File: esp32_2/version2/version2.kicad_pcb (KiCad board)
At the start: 4 copper layers, 31 x 38.5 mm, 30 parts, among them J1 USB_C_Receptacle_USB2.0_16P, J2 Conn_01x08_Pin, J3 Conn_01x08_Pin, SW1 SW_Push, SW2 SW_Push, U1 USBLC6-2SC6, U2 AP2112K-3.3, U3 ESP32-C3-WROOM-02, Y1 Crystal

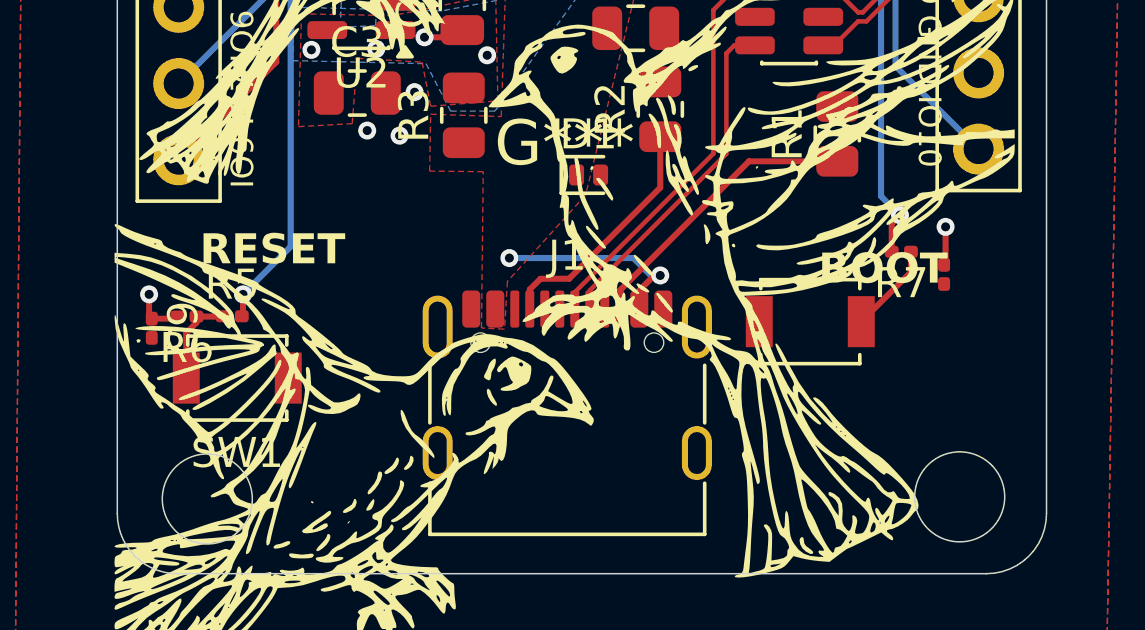
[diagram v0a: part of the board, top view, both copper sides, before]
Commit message: oops some formatting stuff
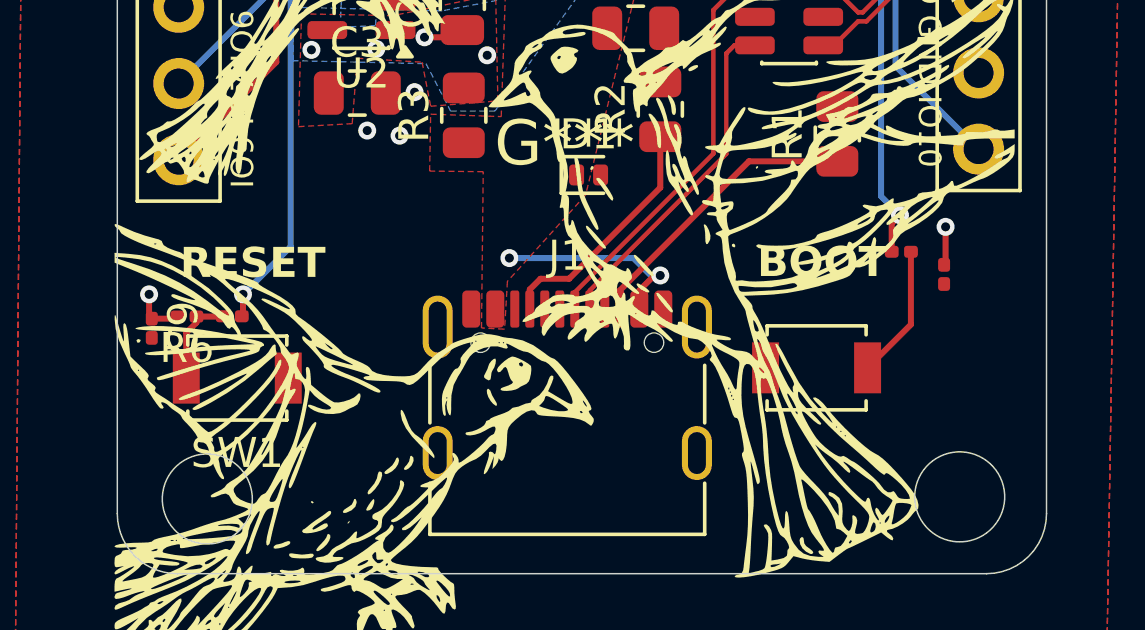
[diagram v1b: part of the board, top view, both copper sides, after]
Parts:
- moved SW2 1.55 mm to (95.8, 80.7)
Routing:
- net IO9: track 46.7 -> 48.1 mm
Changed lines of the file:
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@@
 	(footprint "Button_Switch_SMD:SW_SPST_B3U-1000P"
 		(layer "F.Cu")
-		(at 95.6 79.12)
+		(at 95.81 80.66)
 		(descr "Ultra-small-sized Tactile Switch with High Contact Reliability, Top-actuated Model, without Ground Terminal, without Boss")
 		(tags "Tactile Switch")
@@
 			(at 0 -1.05 0)
 			(layer "F.SilkS")
+			(hide yes)
 			(effects
 				(font
@@
 			(at 0 -1.05 0)
 			(layer "F.SilkS")
+			(hide yes)
 			(effects
 				(font
@@
 	)
 	(gr_text "RESET"
-		(at 75.249801 77.296137 0)
+		(at 74.59 77.75 0)
 		(layer "F.SilkS")
 		(effects
@@
 	)
 	(gr_text "BOOT"
-		(at 95.869635 77.940696 0)
+		(at 93.83 77.72 0)
 		(layer "F.SilkS")
 		(effects
@@
 	)
 	(segment
-		(start 98.955 76.79)
-		(end 98.955 77.465)
+		(start 77.8 60.96)
+		(end 78.56 60.2)
 		(width 0.2)
 		(layer "F.Cu")
@@
 	)
 	(segment
-		(start 77.8 60.96)
-		(end 78.56 60.2)
+		(start 78.56 60.2)
+		(end 78.99 60.2)
 		(width 0.2)
 		(layer "F.Cu")
@@
 	)
 	(segment
-		(start 78.56 60.2)
-		(end 78.99 60.2)
+		(start 98.955 79.215)
+		(end 97.51 80.66)
 		(width 0.2)
 		(layer "F.Cu")
@@
 	)
 	(segment
-		(start 74.546145 73.722333)
-		(end 77.8 70.468478)
+		(start 98.955 76.79)
+		(end 98.955 79.215)
 		(width 0.2)
 		(layer "F.Cu")
@@
 	)
 	(segment
-		(start 100.11 75.96)
-		(end 100.11 77.175)
+		(start 74.546145 73.722333)
+		(end 77.8 70.468478)
 		(width 0.2)
 		(layer "F.Cu")
@@
 	)
 	(segment
-		(start 98.955 77.465)
-		(end 97.3 79.12)
+		(start 100.11 75.96)
+		(end 100.11 77.175)
 		(width 0.2)
 		(layer "F.Cu")
